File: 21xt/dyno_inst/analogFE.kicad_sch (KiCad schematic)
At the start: 20 parts, among them U10 ADA4945-1ACPZ-R2, U14 ADA4945-1ACPZ-R2

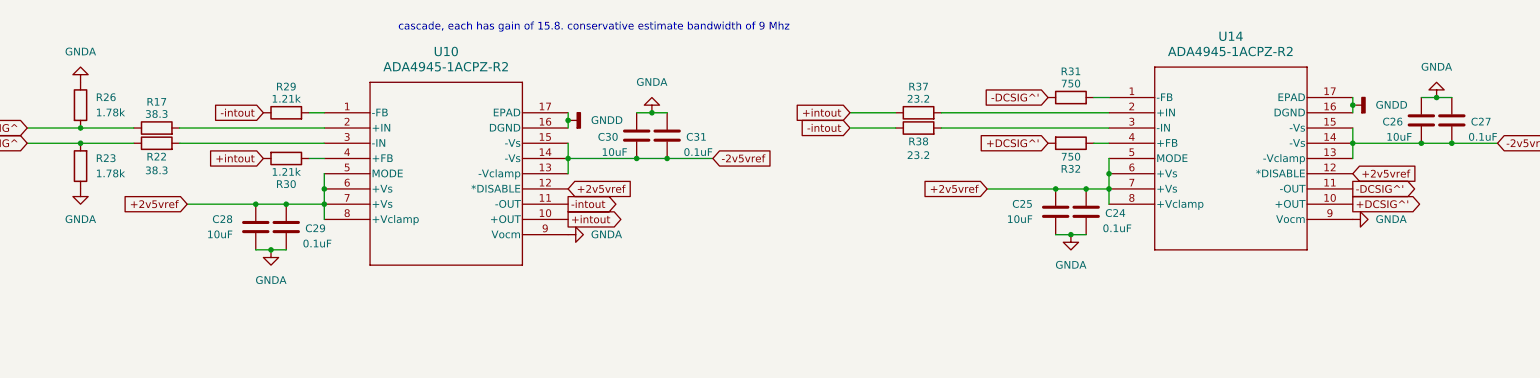
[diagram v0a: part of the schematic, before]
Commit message: sad
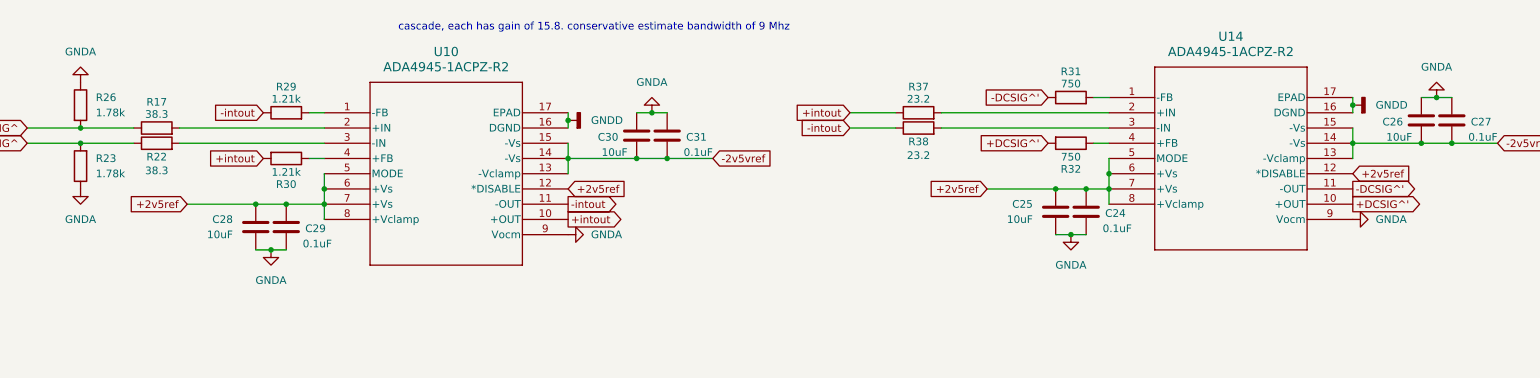
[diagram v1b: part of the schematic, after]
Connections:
- net +2v5vref renamed +2v5ref
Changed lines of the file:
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@@
 		)
 	)
-	(global_label "+2v5vref"
+	(global_label "+2v5ref"
 		(shape input)
 		(at 184.15 68.58 180)
@@
 		)
 		(property "Intersheetrefs" "${INTERSHEET_REFS}"
-			(at 172.6377 68.58 0)
+			(at 173.6053 68.58 0)
 			(effects
 				(font
@@
 		)
 	)
-	(global_label "+2v5vref"
+	(global_label "+2v5ref"
 		(shape input)
 		(at 245.11 66.04 0)
@@
 		)
 		(property "Intersheetrefs" "${INTERSHEET_REFS}"
-			(at 256.6223 66.04 0)
+			(at 255.6547 66.04 0)
 			(effects
 				(font
@@
 		)
 	)
-	(global_label "+2v5vref"
+	(global_label "+2v5ref"
 		(shape input)
 		(at 50.8 71.12 180)
@@
 		)
 		(property "Intersheetrefs" "${INTERSHEET_REFS}"
-			(at 39.2877 71.12 0)
+			(at 40.2553 71.12 0)
 			(effects
 				(font
@@
 		)
 	)
-	(global_label "+2v5vref"
+	(global_label "+2v5ref"
 		(shape input)
 		(at 114.3 68.58 0)
@@
 		)
 		(property "Intersheetrefs" "${INTERSHEET_REFS}"
-			(at 125.8123 68.58 0)
+			(at 124.8447 68.58 0)
 			(effects
 				(font

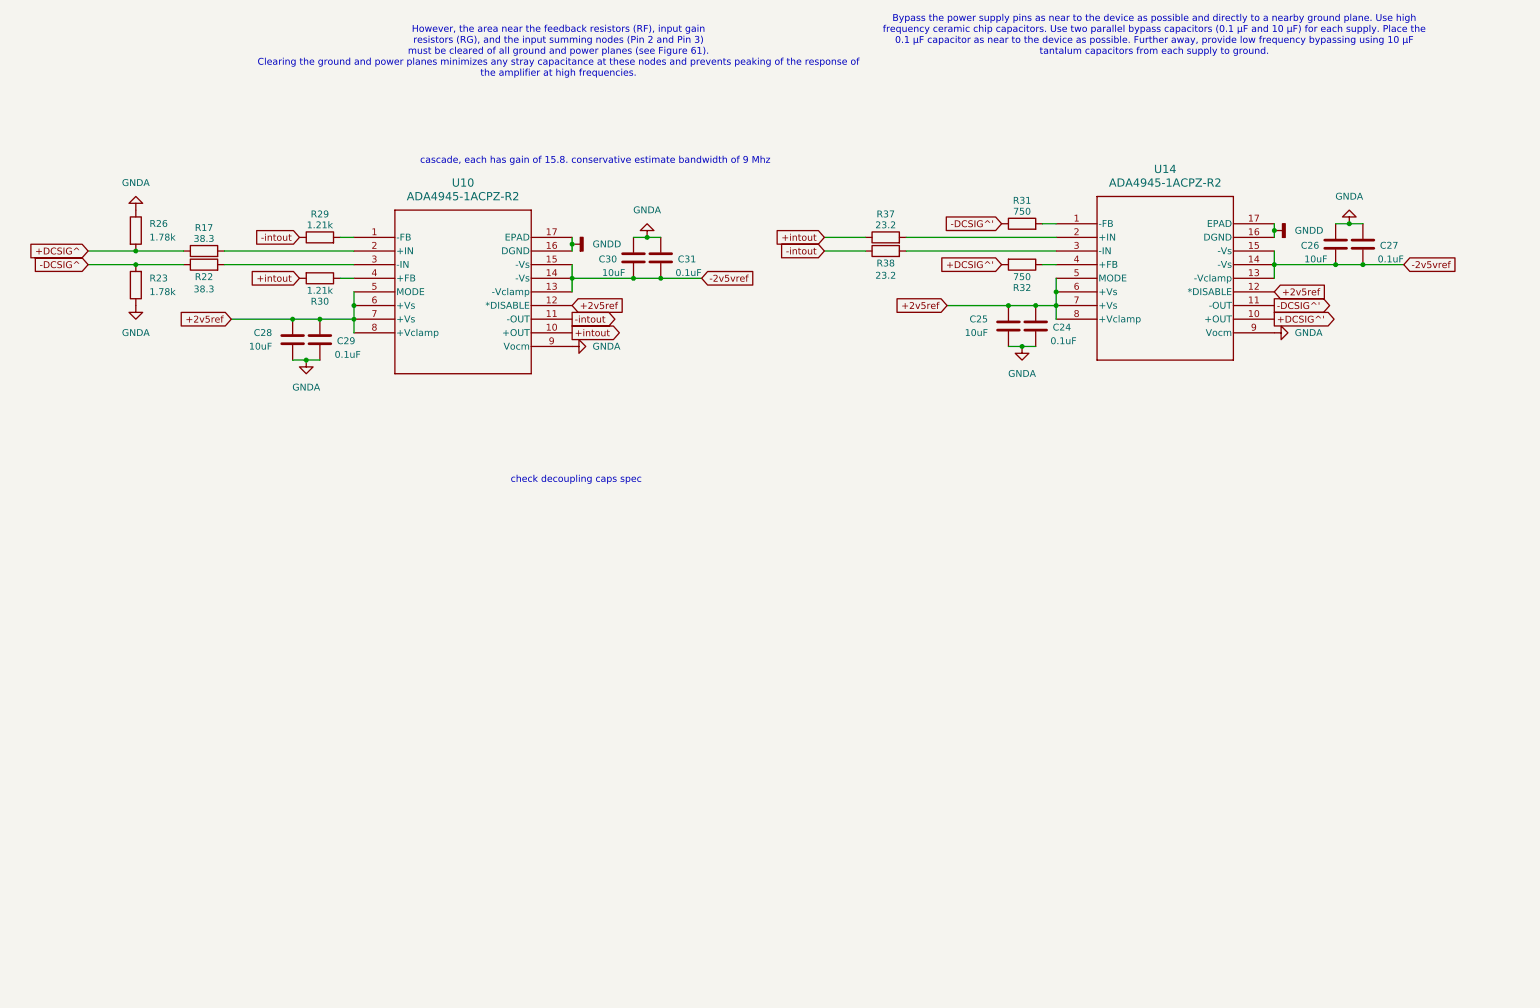
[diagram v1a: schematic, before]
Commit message: sche
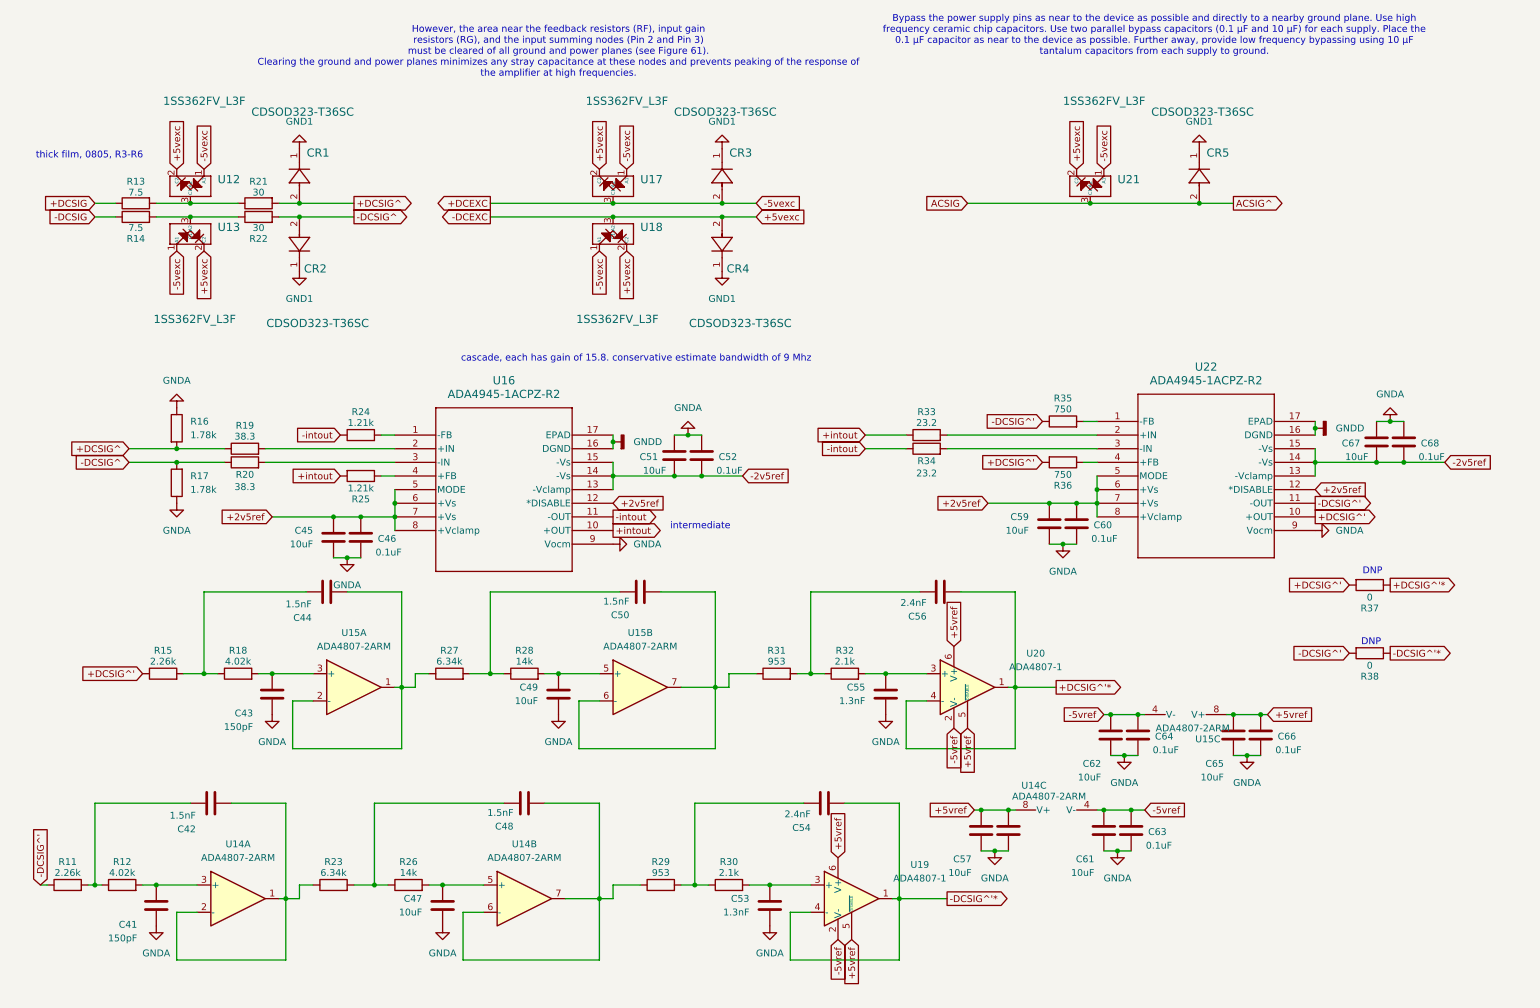
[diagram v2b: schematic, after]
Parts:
- added C41, C43: 150pF, symbol Device:C
- added C42, C44, C48, C50: 1.5nF, symbol Device:C
- added C47, C49, C57, C61, C62, C65: 10uF, symbol Device:C
- added C53, C55: 1.3nF, symbol Device:C
- added C54, C56: 2.4nF, symbol Device:C
- added C58, C63, C64, C66: 0.1uF, symbol Device:C
- added CR1, CR2, CR3, CR4, CR5: CDSOD323-T36SC, DIODE_CDSOD323-T36SC_BRN, symbol dyno_inst_sym:CDSOD323-T36SC
- added R11, R15: 2.26k, symbol Device:R
- added R12, R18: 4.02k, symbol Device:R
- added R13, R14: 7.5, symbol Device:R
- added R21, R22: 30, symbol Device:R
- added R23, R27: 6.34k, symbol Device:R
- added R26, R28: 14k, symbol Device:R
- added R29, R31: 953, symbol Device:R
- added R30, R32: 2.1k, symbol Device:R
- added R37, R38: 0, symbol Device:R
- added U12, U13, U17, U18, U21: 1SS362FV_L3F, SOT-723 VESM_TOS, symbol dyno_inst_sym:1SS362FV_L3F
- added U14, U15: ADA4807-2ARM, Package_SO:MSOP-8_3x3mm_P0.65mm, symbol Amplifier_Operational:ADA4807-2ARM
- added U19, U20: ADA4807-1, symbol Amplifier_Operational:ADA4807-1
- U16: renamed from U10; footprint LFCSP16_ADA4945-1ACPZ-R2_ADI -> dynoinst_fp:LFCSP16_ADA4945-1ACPZ-R2_ADI
- U22: renamed from U14; footprint LFCSP16_ADA4945-1ACPZ-R2_ADI -> dynoinst_fp:LFCSP16_ADA4945-1ACPZ-R2_ADI
- renumbered C28 to C45, C29 to C46, C30 to C51, C31 to C52, C25 to C59, C24 to C60, C26 to C67, C27 to C68, R26 to R16, R23 to R17, R17 to R19, R22 to R20, R29 to R24, R30 to R25, R37 to R33, R38 to R34, R31 to R35, R32 to R36
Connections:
- net +DCSIG^: now also CR1.2, R21.2
- net +DCSIG^': now also R15.1, R37.2
- net -DCSIG^: now also CR2.2, R22.2
- net -DCSIG^': now also R11.1, R38.2
- net GNDA: now also C41.2, C43.2, C47.2, C49.2, C53.2, C55.2, C57.2, C58.2, C61.2, C62.2, C63.2, C64.2, C65.2, C66.2
- net -2v5vref renamed -2v5ref
- new net: C42.2, R23.1, U14.1, U14.2 (-)
- new net: C41.1, R12.2, U14.3 (+)
- new net: C48.1, R23.2, R26.1
- new net: C47.1, R26.2, U14.5 (+)
- new net: C50.1, R27.2, R28.1
- new net: C50.2, R31.1, U15.6 (-), U15.7
- new net: C49.1, R28.2, U15.5 (+)
- new net: R13.2, R21.1, U12.3 (C1/A2)
- new net: R14.2, R22.1, U13.3 (C1/A2)
- new net: C54.1, R29.2, R30.1
- new net: C53.1, R30.2, U19.3 (+)
- new net: C56.1, R31.2, R32.1
- new net: C44.1, R15.2, R18.1
- new net: C44.2, R27.1, U15.1, U15.2 (-)
- new net: C43.1, R18.2, U15.3 (+)
- new net: C55.1, R32.2, U20.3 (+)
- new net: C48.2, R29.1, U14.6 (-), U14.7
- new net: C42.1, R11.2, R12.1
- new net +5vexc: CR4.2, U12.2 (C2), U13.2 (C2), U17.2 (C2), U18.2 (C2), U18.3 (C1/A2), U21.2 (C2)
- new net +5vref: C57.1, C58.1, C65.1, C66.1, U14.8 (V+), U15.8 (V+), U19.5 (~{DISABLE}), U19.6 (V+), U20.5 (~{DISABLE}), U20.6 (V+)
- new net +DCEXC: CR3.2, U12.1 (A1), U13.1 (A1), U17.1 (A1), U17.3 (C1/A2), U18.1 (A1), U21.1 (A1)
- new net +DCSIG: R13.1
- new net +DCSIG^'*: C56.2, R37.1, U20.1, U20.4 (-)
- new net -5vref: C61.1, C62.1, C63.1, C64.1, U14.4 (V-), U15.4 (V-), U19.2 (V-), U20.2 (V-)
- new net -DCSIG: R14.1
- new net -DCSIG^'*: C54.2, R38.1, U19.1, U19.4 (-)
- new net ACSIG: CR5.2, U21.3 (C1/A2)
- new net GND1: CR1.1, CR2.1, CR3.1, CR4.1, CR5.1
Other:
- note added: "DNP"
- note added: "intermediate"
- note added: "thick film, 0805, R3-R6"
- note removed: "check decoupling caps spec"
- moved on the sheet: C45, C46, C51, C52, C59, C60, C67, C68, R16, R17, R19, R20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
